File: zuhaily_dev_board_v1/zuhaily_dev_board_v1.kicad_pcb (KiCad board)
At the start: 2 copper layers, 56 parts, among them J1 USB_B_Micro, J2 Micro_SD_Card, J3 DC_JACK, J4 Conn_01x32_Female, Q1 FS8205A, Q2 FDN340P, SW1 SW_DPDT_x2, SW2 SW_SPST, SW3 SW_DIP_x04, SW4 SW_DIP_x04, SW5 SW_DIP_x04, U1 74LVC245, U10 DW-01, U2 LM1117-5.0, U3 CH340G, U4 LM1117-3.3, U5 ATmega328-PU, U7 TP4056, U8 LMV358, Y1 Crystal_12MHz, Y2 Crystal_16MHz

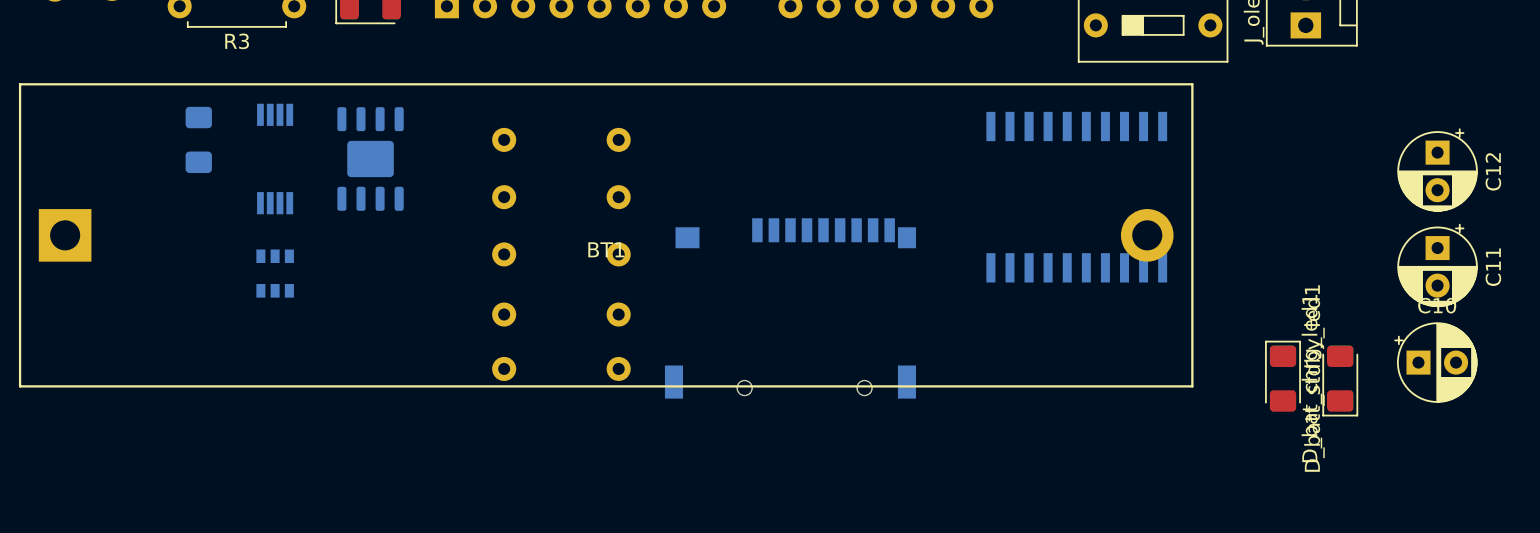
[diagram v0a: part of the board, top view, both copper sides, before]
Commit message: added images
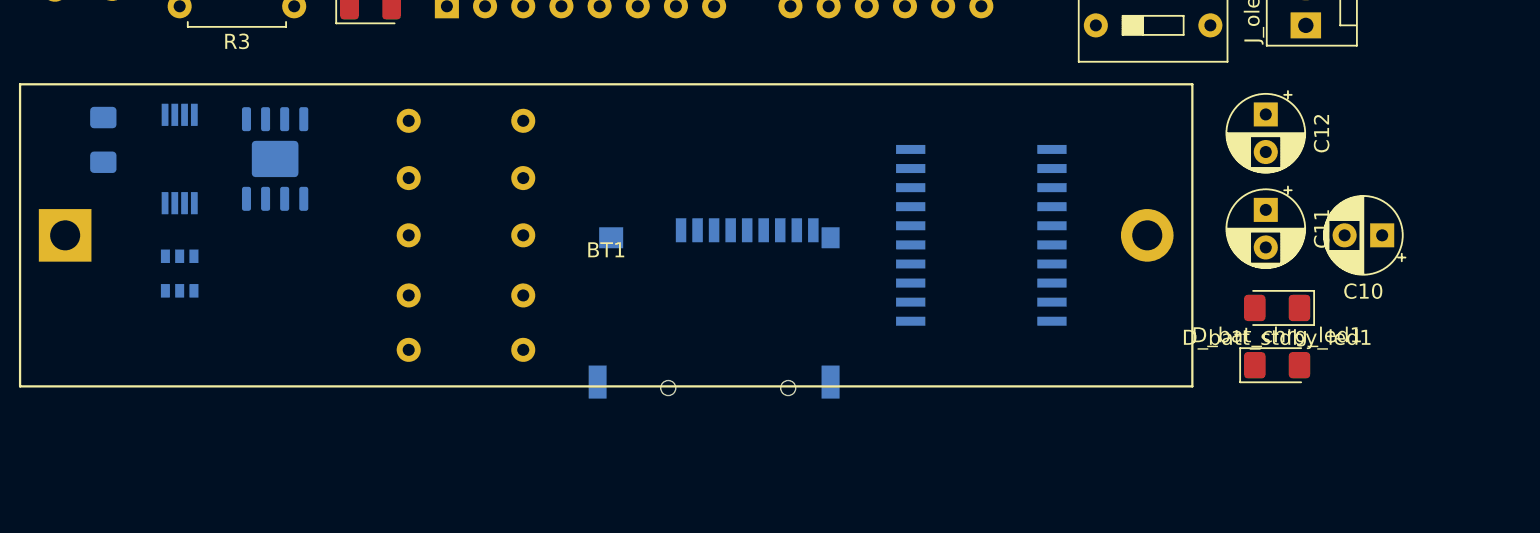
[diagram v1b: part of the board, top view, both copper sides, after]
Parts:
- moved C12 11.7 mm to (137.0, 116.4)
- moved C11 11.7 mm to (137.0, 122.8)
- moved C10 8.80 mm to (144.8, 124.5), turned to 180 degrees
- moved U1 6.84 mm to (118.1, 124.5), turned to 180 degrees
- moved R7 6.48 mm to (87.6, 124.5)
- moved R8 6.48 mm to (87.6, 128.5)
- moved R12 6.48 mm to (80.0, 120.7)
- moved R13 6.48 mm to (80.0, 116.8)
- moved R14 6.48 mm to (80.0, 132.1)
- moved D3 6.35 mm to (59.7, 118.1)
- moved Q1 6.35 mm to (64.8, 119.4)
- moved U10 6.35 mm to (64.8, 127.0)
- moved U7 6.35 mm to (71.1, 119.4)
- moved J2 5.08 mm to (100.3, 134.6)
- moved D_bat_chrg_led1 4.71 mm to (137.8, 129.3), turned to 180 degrees
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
